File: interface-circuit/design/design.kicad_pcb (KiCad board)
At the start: 2 copper layers, 23 parts, among them J10 FAN_RELAY, J11 Conn_Switch, J12 Conn_Reset, J2 Screw_Term_RPi, J3 Screw_Term_Detector, J4 12V_IN, J5 Conn_Pwr_LED, J6 Conn_Piezo, J7 Conn_Printer_Mode, J8 Conn_Fan_Mode, J9 PRINTER_RELAY, Q1 2N3904-AP, Q2 2N3904-AP, Q3 2N3904-AP, U1 LogicLevelConverter_BOB-08745

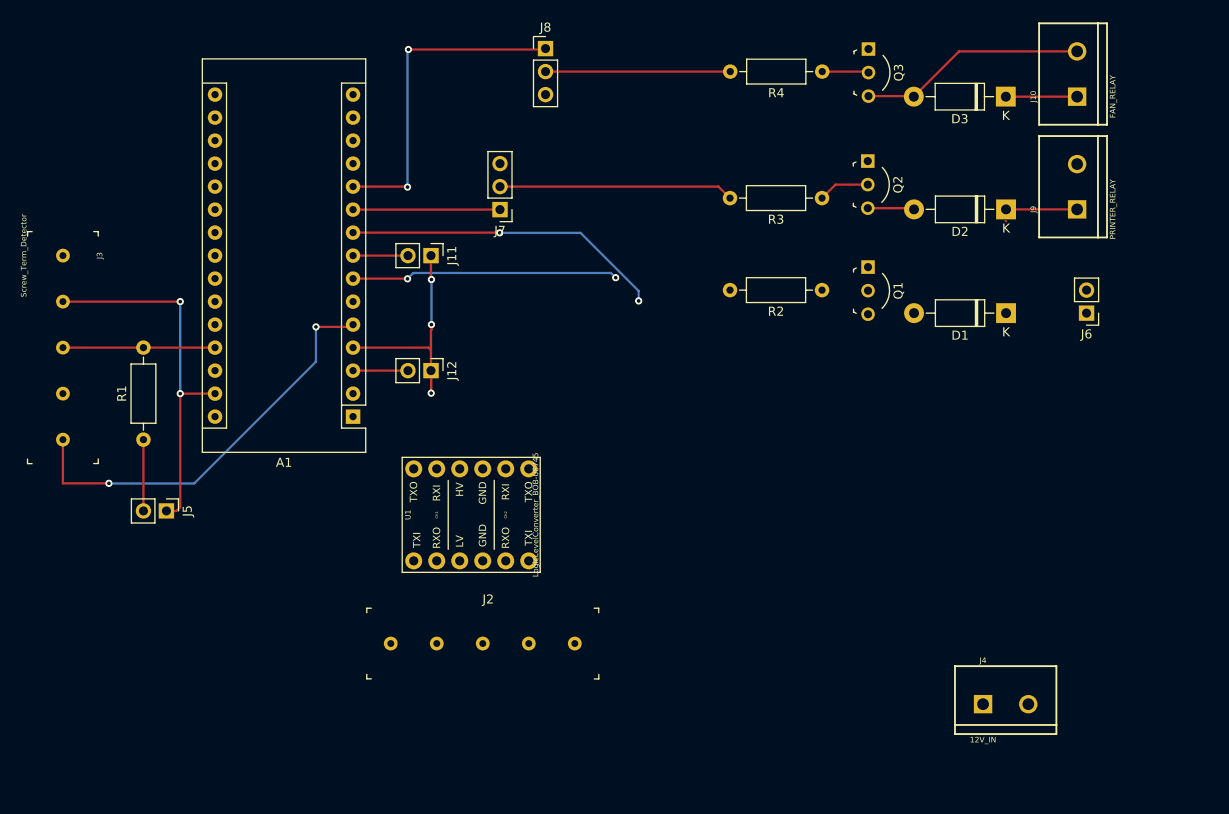
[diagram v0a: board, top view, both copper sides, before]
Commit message: Done with manual routing
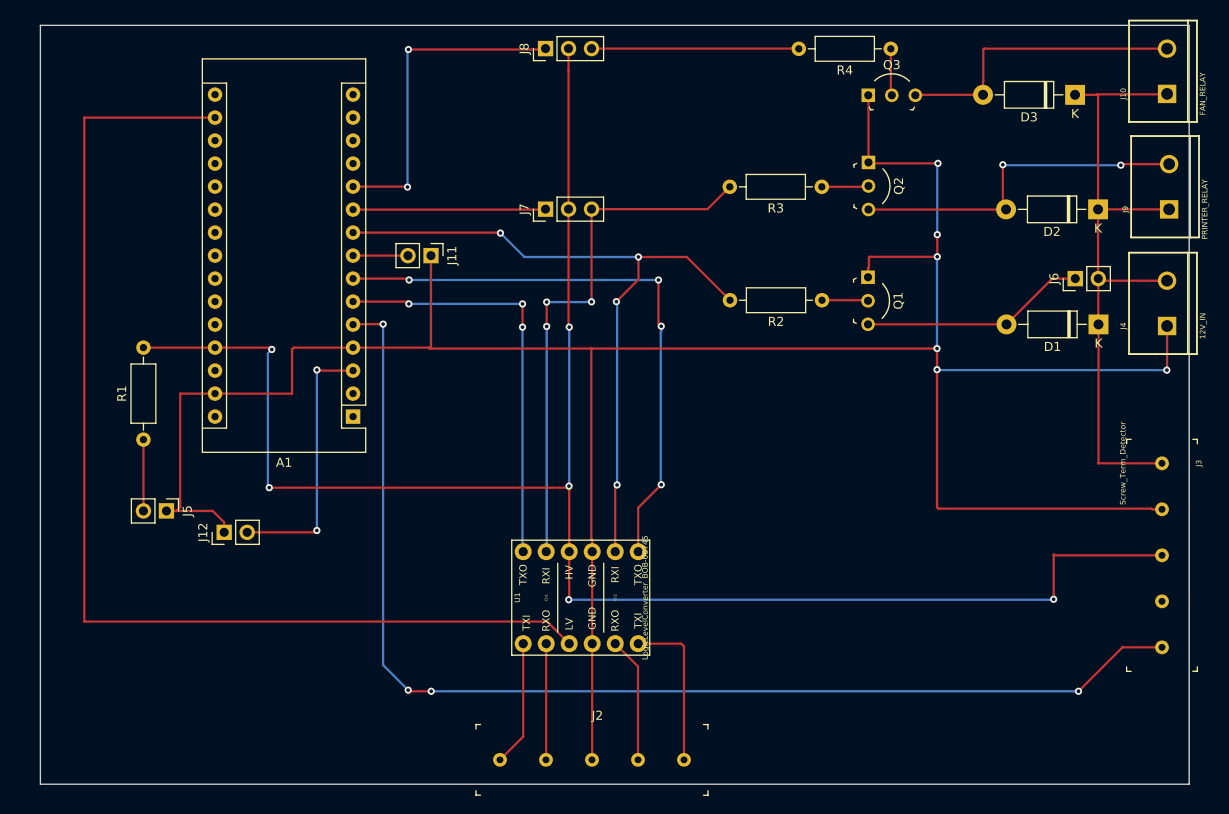
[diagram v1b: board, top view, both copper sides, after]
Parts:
- moved J3 123.5 mm to (146.8, 124.5)
- moved J4 46.4 mm to (147.3, 109.4), turned to 90 degrees
- moved J12 29.0 mm to (43.2, 132.2), turned to 90 degrees
- moved J2 17.6 mm to (73.7, 157.3)
- moved U1 15.2 mm to (82.6, 139.4)
- moved D1 10.3 mm to (139.8, 109.2)
- moved D2 10.2 mm to (139.7, 96.5)
- moved J9 10.2 mm to (147.5, 96.5)
- moved J10 9.94 mm to (147.3, 83.7)
- moved R4 7.98 mm to (116.8, 78.8)
- moved D3 7.65 mm to (137.2, 83.8)
- moved Q3 5.11 mm to (114.3, 83.9), turned to 0 degrees
- moved J7 5.03 mm to (78.7, 96.5), turned to 90 degrees
- moved J6 4.01 mm to (137.2, 104.1), turned to 90 degrees
- moved R3 1.24 mm to (109.2, 94.0)
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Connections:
- J2 pad 1: /LV_PrinterPowerStatus -> /LV_PrinterPowerDemand
- J2 pad 2: /LV_PrinterPowerDemand -> /LV_PrinterPowerStatus
- J2 pad 4: /LV_FanPowerDemand -> /LV_AlarmTriggered
- J2 pad 5: /LV_AlarmTriggered -> /LV_FanPowerDemand
- J7 pad 2: /HV_PrinterPowerStatus -> +5V
- J7 pad 3: +5V -> /HV_PrinterPowerStatus
- J8 pad 2: /SW_FAN_RELAY -> +5V
- J8 pad 3: +5V -> /SW_FAN_RELAY
- U1 pad 1: /LV_FanPowerDemand -> /HV_PrinterPowerStatus
- U1 pad 10: /HV_FanPowerDemand -> /LV_AlarmTriggered
- U1 pad 11: /LV_PrinterPowerStatus -> /HV_PrinterPowerDemand
- U1 pad 12: /LV_AlarmTriggered -> /HV_FanPowerDemand
- U1 pad 2: /LV_FanPowerDemand -> /HV_AlarmTriggered
- U1 pad 3: /HV_PrinterPowerStatus -> /LV_PrinterPowerDemand
- U1 pad 4: /HV_AlarmTriggered -> /LV_FanPowerDemand
- U1 pad 9: /HV_PrinterPowerDemand -> /LV_PrinterPowerStatus
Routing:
- net GND: track 65.5 -> 285.1 mm, vias 5 -> 6
- net +5V: track 16.8 -> 194.1 mm, vias 0 -> 6
- net +3V3: track 0.00 -> 124.6 mm
- net /DETECTOR_SIGNAL: track 46.4 -> 130.6 mm, vias 2 -> 4
- net +12V: track 15.8 -> 73.6 mm
- net /HV_PrinterPowerDemand: track 0.00 -> 46.3 mm, vias 0 -> 3
- net /HV_AlarmTriggered: track 35.3 -> 78.4 mm, vias 2 -> 4
- net /HV_FanPowerDemand: track 29.5 -> 65.0 mm, vias 2 -> 4
- net Net-(D2-Pad2): track 5.16 -> 38.7 mm, vias 0 -> 2
- net /HV_PrinterPowerStatus: track 25.9 -> 59.1 mm, vias 0 -> 3
- net /-PIEZO: track 0.00 -> 25.0 mm
- net /RESET: track 6.06 -> 29.5 mm, vias 0 -> 2
- net /LV_FanPowerDemand: track 0.00 -> 17.7 mm
- net /LV_PrinterPowerDemand: track 0.00 -> 13.9 mm
- net /LV_AlarmTriggered: track 0.00 -> 13.9 mm
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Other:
- board outline added: 126.8 x 83.8 mm
